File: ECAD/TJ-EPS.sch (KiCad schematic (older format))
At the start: 38 parts, among them J1 SWD, J2 BOOT, Q1 2N7002, Q2 IRF7425, U1 CD74HC4067SM, U2 MAX6369, U3 CD74HC4067SM, U4 STM32F103C8Tx, Y1 8MHz

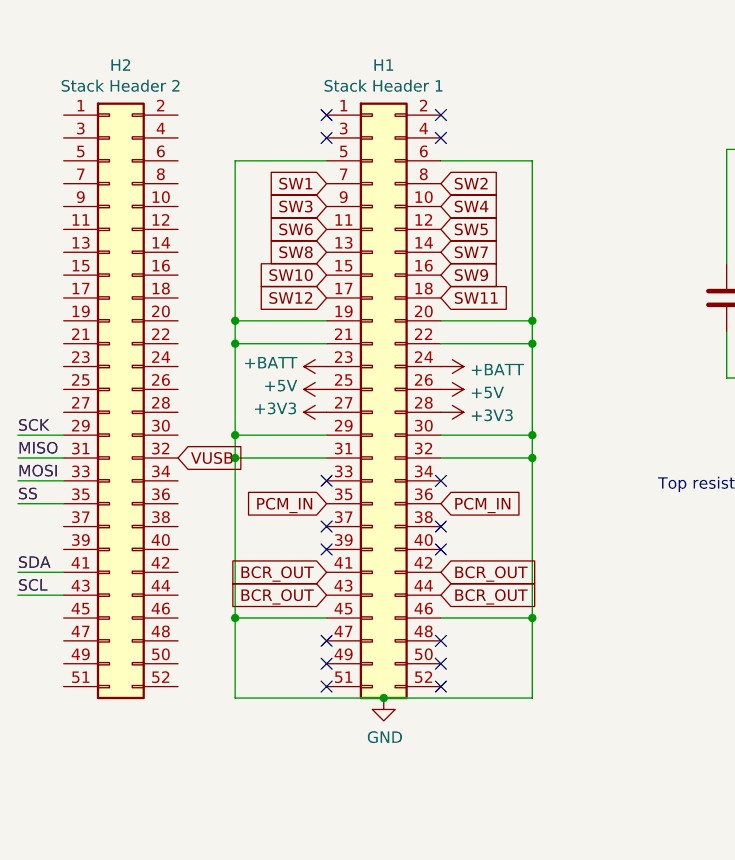
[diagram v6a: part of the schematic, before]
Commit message: Update stack header pinouts and re-annotate
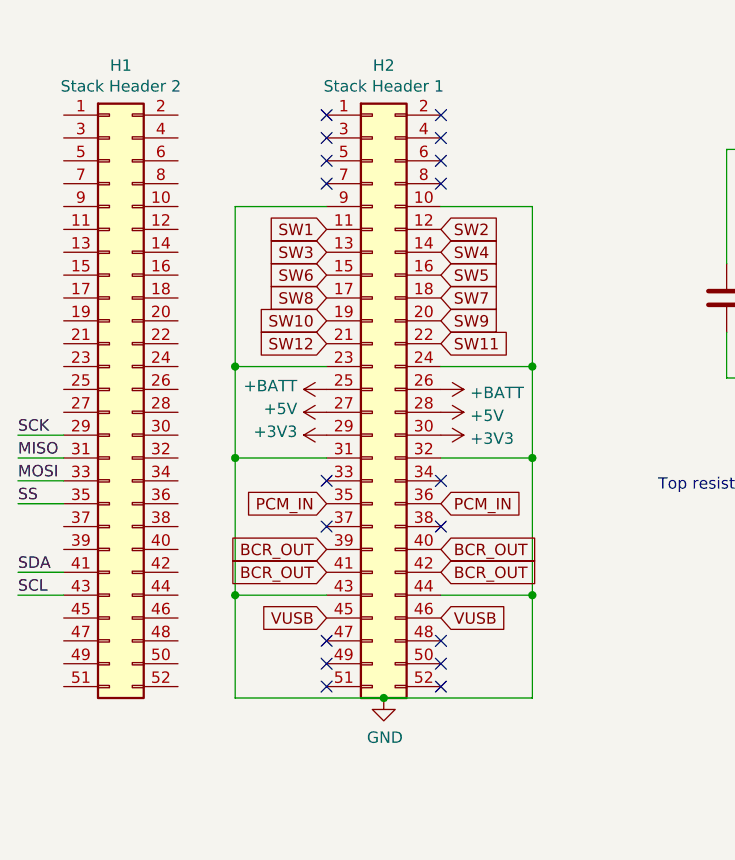
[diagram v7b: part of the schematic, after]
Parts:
- renumbered H2 to H1, H1 to H2
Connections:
- net +3V3: now also H2.29 (Pin_29), H2.30 (Pin_30); no longer H2.27 (Pin_27), H2.28 (Pin_28)
- net +5V: now also H2.27 (Pin_27), H2.28 (Pin_28); no longer H2.25 (Pin_25), H2.26 (Pin_26)
- net +BATT: now also H2.25 (Pin_25), H2.26 (Pin_26); no longer H2.23 (Pin_23), H2.24 (Pin_24)
- net BCR_OUT: now also H2.39 (Pin_39), H2.40 (Pin_40); no longer H2.43 (Pin_43), H2.44 (Pin_44)
- net GND: now also H2.10 (Pin_10), H2.23 (Pin_23), H2.24 (Pin_24), H2.43 (Pin_43), H2.44 (Pin_44), H2.9 (Pin_9); no longer H2.19 (Pin_19), H2.20 (Pin_20), H2.21 (Pin_21), H2.22 (Pin_22), H2.29 (Pin_29), H2.30 (Pin_30), H2.45 (Pin_45), H2.46 (Pin_46), H2.5 (Pin_5), H2.6 (Pin_6)
- net SW1: now also H2.11 (Pin_11); no longer H2.7 (Pin_7)
- net SW10: now also H2.19 (Pin_19); no longer H2.15 (Pin_15)
- net SW11: now also H2.22 (Pin_22); no longer H2.18 (Pin_18)
- net SW12: now also H2.21 (Pin_21); no longer H2.17 (Pin_17)
- net SW2: now also H2.12 (Pin_12); no longer H2.8 (Pin_8)
- net SW3: now also H2.13 (Pin_13); no longer H2.9 (Pin_9)
- net SW4: now also H2.14 (Pin_14); no longer H2.10 (Pin_10)
- net SW5: now also H2.16 (Pin_16); no longer H2.12 (Pin_12)
- net SW6: now also H2.15 (Pin_15); no longer H2.11 (Pin_11)
- net SW7: now also H2.18 (Pin_18); no longer H2.14 (Pin_14)
- net SW8: now also H2.17 (Pin_17); no longer H2.13 (Pin_13)
- net SW9: now also H2.20 (Pin_20); no longer H2.16 (Pin_16)
- net VUSB: now also H2.45 (Pin_45), H2.46 (Pin_46); no longer H1.32 (Pin_32)
- no-connect marks 16 -> 18

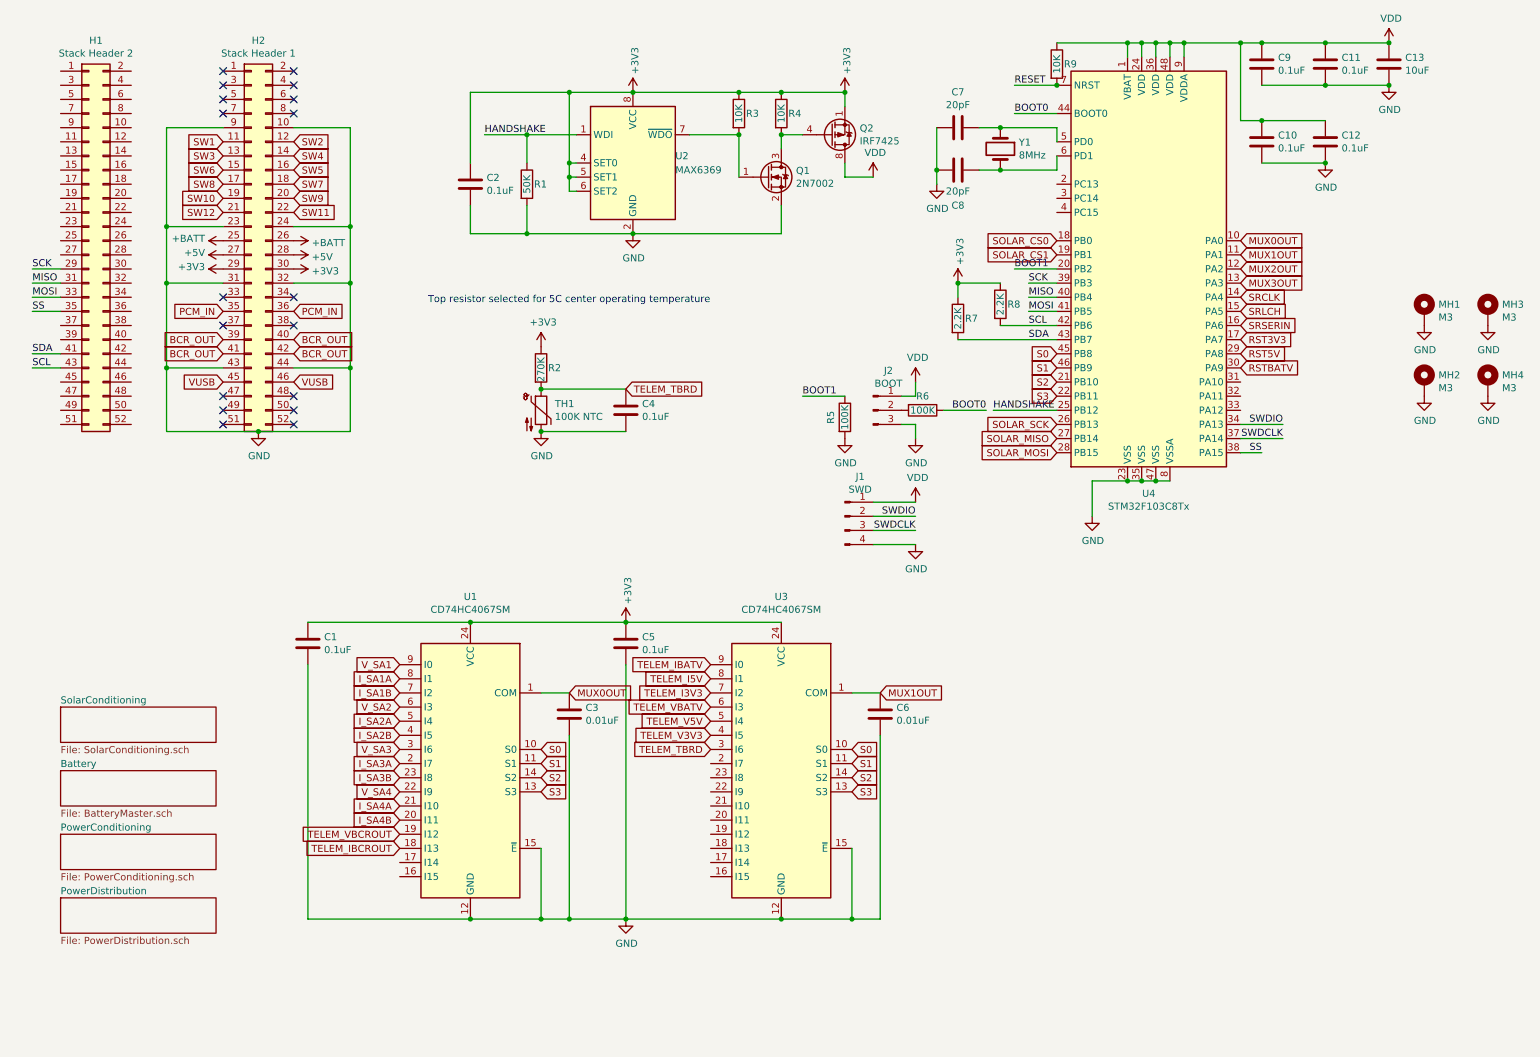
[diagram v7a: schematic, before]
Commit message: Condense muxes and add srrst
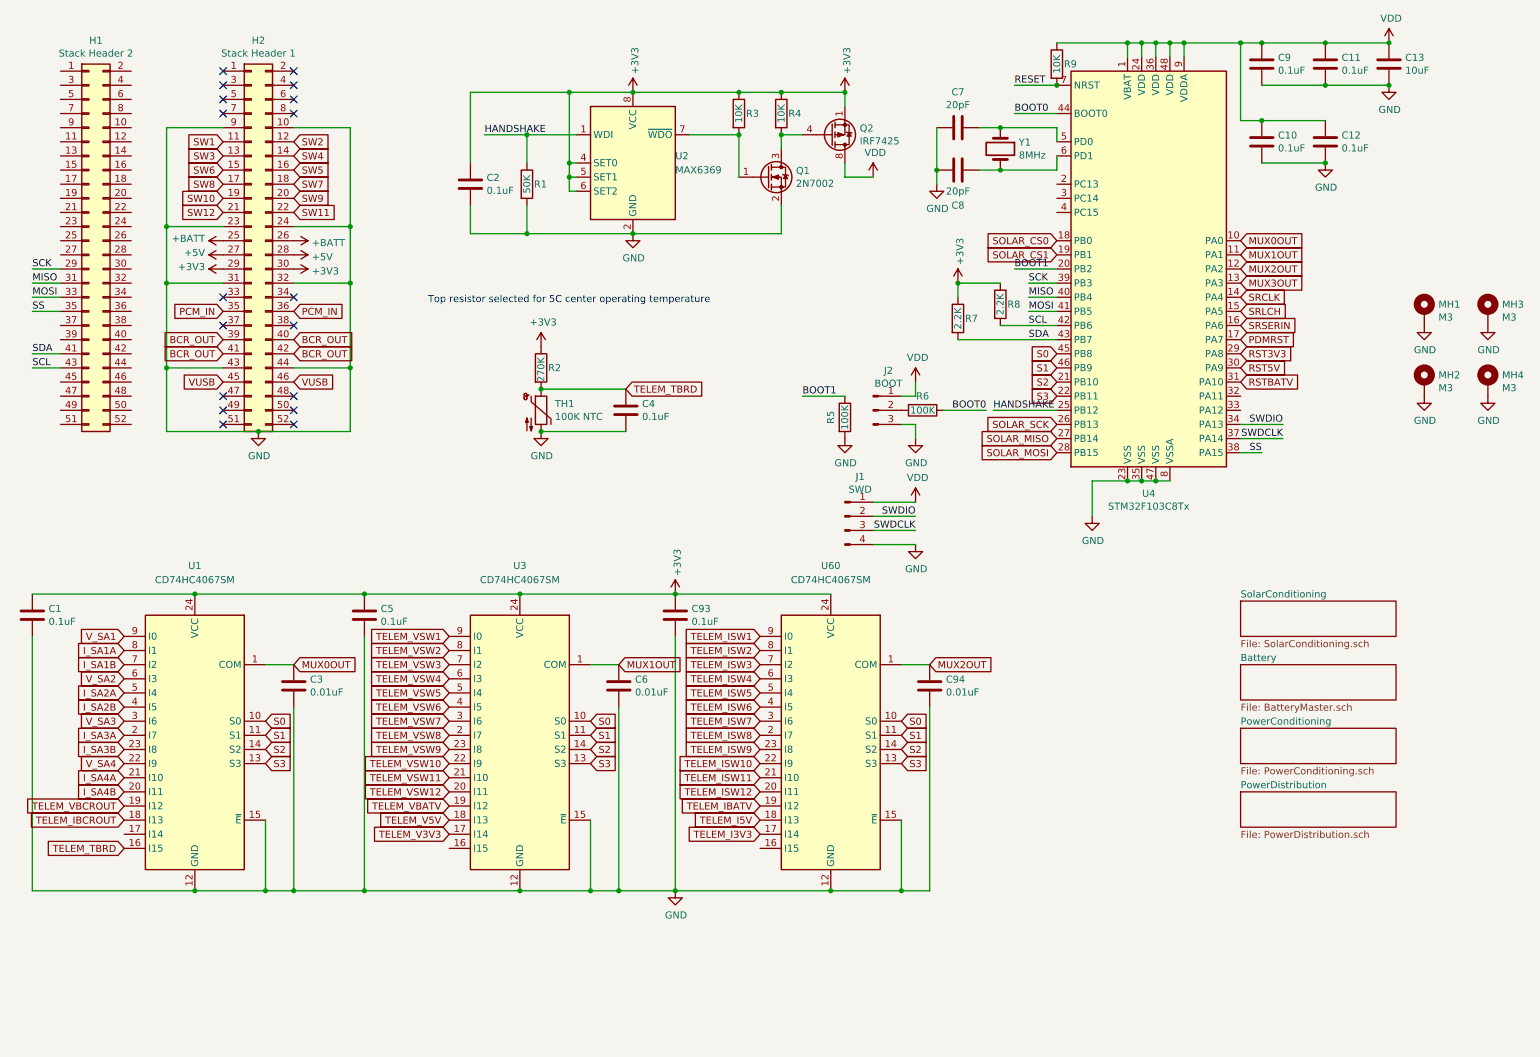
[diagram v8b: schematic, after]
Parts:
- added C93: 0.1uF, Capacitor_SMD:C_0805_2012Metric, symbol Device:C
- added C94: 0.01uF, Capacitor_SMD:C_0805_2012Metric, symbol Device:C
- added U60: CD74HC4067SM, Package_SO:SSOP-24_5.3x8.2mm_P0.65mm, symbol 74xx:CD74HC4067SM
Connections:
- net +3V3: now also C93.1, U60.24 (VCC)
- net GND: now also C93.2, C94.2, U60.12 (GND), U60.15 (~E)
- net MUX2OUT: now also C94.1, U60.1 (COM)
- net RST3V3: now also U4.29 (PA8); no longer U4.17 (PA7)
- net RST5V: now also U4.30 (PA9); no longer U4.29 (PA8)
- net RSTBATV: now also U4.31 (PA10); no longer U4.30 (PA9)
- net S0: now also U60.10 (S0)
- net S1: now also U60.11 (S1)
- net S2: now also U60.14 (S2)
- net S3: now also U60.13 (S3)
- net TELEM_I3V3: now also U60.17 (I14); no longer U3.7 (I2)
- net TELEM_I5V: now also U60.18 (I13); no longer U3.8 (I1)
- net TELEM_IBATV: now also U60.19 (I12); no longer U3.9 (I0)
- net TELEM_TBRD: now also U1.16 (I15); no longer U3.3 (I6)
- net TELEM_V3V3: now also U3.17 (I14); no longer U3.4 (I5)
- net TELEM_V5V: now also U3.18 (I13); no longer U3.5 (I4)
- net TELEM_VBATV: now also U3.19 (I12); no longer U3.6 (I3)
- net TELEM_VSW8: now reaches U3.2 (I7)
- net TELEM_VSW12: now reaches U3.20 (I11)
- net TELEM_VSW11: now reaches U3.21 (I10)
- net TELEM_VSW10: now reaches U3.22 (I9)
- net TELEM_VSW9: now reaches U3.23 (I8)
- new net PDMRST: U4.17 (PA7)
- new net TELEM_ISW1: U60.9 (I0)
- new net TELEM_ISW10: U60.22 (I9)
- new net TELEM_ISW11: U60.21 (I10)
- new net TELEM_ISW12: U60.20 (I11)
- new net TELEM_ISW2: U60.8 (I1)
- new net TELEM_ISW3: U60.7 (I2)
- new net TELEM_ISW4: U60.6 (I3)
- new net TELEM_ISW5: U60.5 (I4)
- new net TELEM_ISW6: U60.4 (I5)
- new net TELEM_ISW7: U60.3 (I6)
- new net TELEM_ISW8: U60.2 (I7)
- new net TELEM_ISW9: U60.23 (I8)
- new net TELEM_VSW1: U3.9 (I0)
- new net TELEM_VSW2: U3.8 (I1)
- new net TELEM_VSW3: U3.7 (I2)
- new net TELEM_VSW4: U3.6 (I3)
- new net TELEM_VSW5: U3.5 (I4)
- new net TELEM_VSW6: U3.4 (I5)
- new net TELEM_VSW7: U3.3 (I6)
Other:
- moved on the sheet: C1, C3, U1
